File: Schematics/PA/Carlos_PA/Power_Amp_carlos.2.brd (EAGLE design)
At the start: 70.2 x 70.2 mm, 107 parts, among them J1 4_PIN_AMPCONN, U1 LME49830, U2 LME49830, U3 LME49830

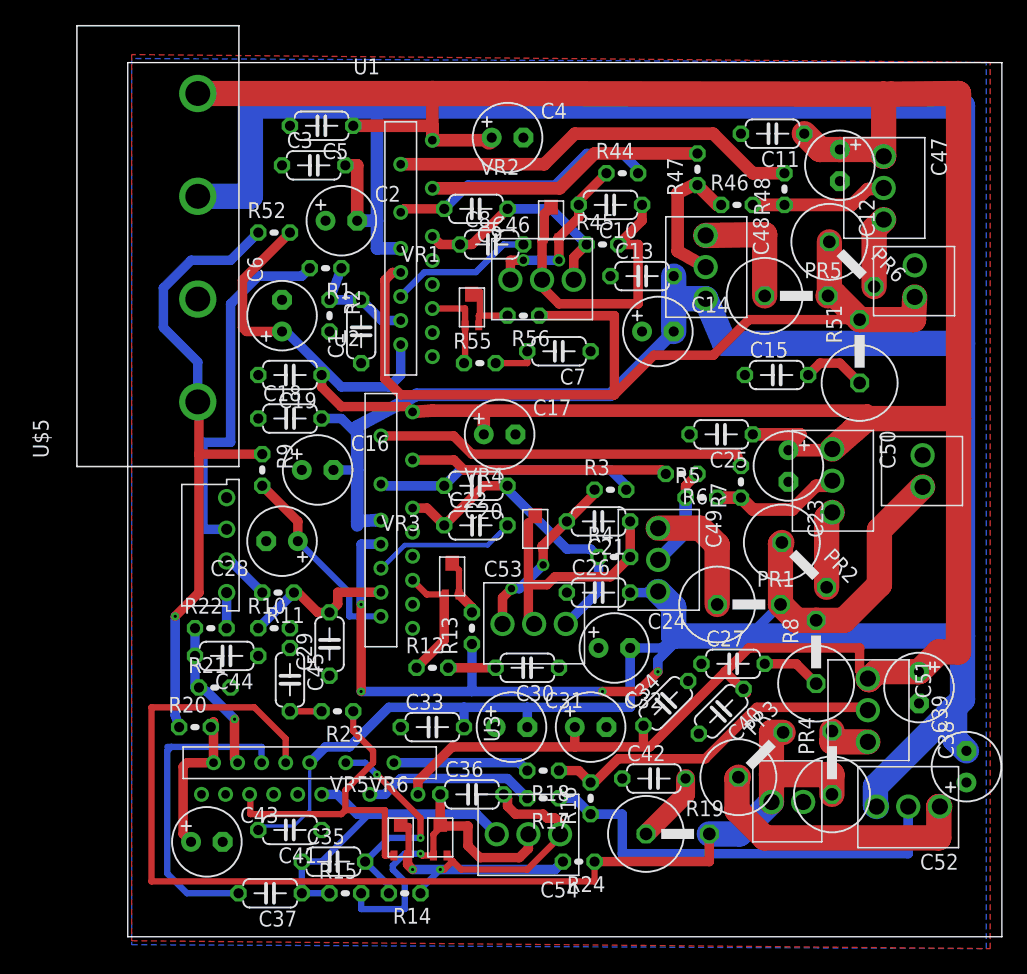
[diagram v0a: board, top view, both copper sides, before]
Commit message: updating to master
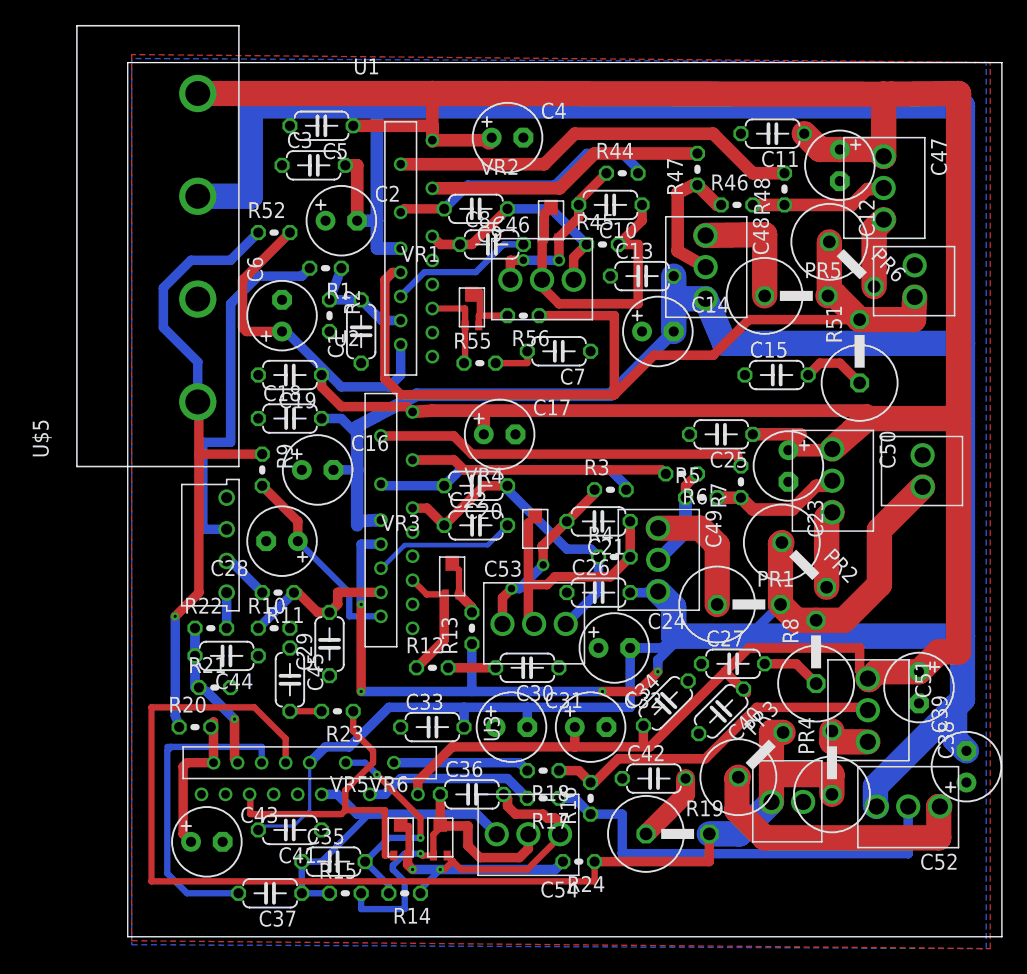
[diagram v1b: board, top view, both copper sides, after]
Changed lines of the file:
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@@
 <setting verticaltext="up"/>
 </settings>
-<grid distance="0.003125" unitdist="mic" unit="inch" style="lines" multiple="1" display="no" altdistance="0.025" altunitdist="inch" altunit="inch"/>
+<grid distance="0.01" unitdist="inch" unit="inch" style="lines" multiple="1" display="yes" altdistance="0.025" altunitdist="inch" altunit="inch"/>
 <layers>
-<layer number="1" name="Top" color="4" fill="1" visible="yes" active="yes"/>
+<layer number="1" name="Top" color="4" fill="1" visible="no" active="yes"/>
 <layer number="16" name="Bottom" color="1" fill="1" visible="yes" active="yes"/>
 <layer number="17" name="Pads" color="2" fill="1" visible="yes" active="yes"/>
@@
 <layer number="19" name="Unrouted" color="6" fill="1" visible="yes" active="yes"/>
 <layer number="20" name="Dimension" color="15" fill="1" visible="yes" active="yes"/>
-<layer number="21" name="tPlace" color="7" fill="1" visible="yes" active="yes"/>
+<layer number="21" name="tPlace" color="7" fill="1" visible="no" active="yes"/>
 <layer number="22" name="bPlace" color="7" fill="1" visible="yes" active="yes"/>
 <layer number="23" name="tOrigins" color="15" fill="1" visible="yes" active="yes"/>
 <layer number="24" name="bOrigins" color="15" fill="1" visible="yes" active="yes"/>
-<layer number="25" name="tNames" color="7" fill="1" visible="yes" active="yes"/>
+<layer number="25" name="tNames" color="7" fill="1" visible="no" active="yes"/>
 <layer number="26" name="bNames" color="7" fill="1" visible="yes" active="yes"/>
 <layer number="27" name="tValues" color="7" fill="1" visible="no" active="yes"/>
@@
 </class>
 </classes>
-<designrules name="default">
-<description language="de">&lt;b&gt;EAGLE Design Rules&lt;/b&gt;
+<designrules name="epl-lpkf">
+<description language="en">&lt;b&gt;EAGLE Design Rules for PSU Electronics Prototyping Lab&lt;/b&gt;
 &lt;p&gt;
-Die Standard-Design-Rules sind so gewählt, dass sie für
-die meisten Anwendungen passen. Sollte ihre Platine
-besondere Anforderungen haben, treffen Sie die erforderlichen
-Einstellungen hier und speichern die Design Rules unter
-einem neuen Namen ab.</description>
-<description language="en">&lt;b&gt;EAGLE Design Rules&lt;/b&gt;
-&lt;p&gt;
-The default Design Rules have been set to cover
-a wide range of applications. Your particular design
-may have different requirements, so please make the
-necessary adjustments and save your customized
-design rules under a new name.</description>
+2013-03-03: Modified from  &lt;b&gt;sunstone_quickturn.dru&lt;/b&gt; to meet minimum drills and spacing for the LPKF S63 Circuit Board Router.
+&lt;/p&gt;</description>
 <param name="layerSetup" value="(1*16)"/>
-<param name="mtCopper" value="0.035mm 0.035mm 0.035mm 0.035mm 0.035mm 0.035mm 0.035mm 0.035mm 0.035mm 0.035mm 0.035mm 0.035mm 0.035mm 0.035mm 0.035mm 0.035mm"/>
-<param name="mtIsolate" value="1.5mm 0.15mm 0.2mm 0.15mm 0.2mm 0.15mm 0.2mm 0.15mm 0.2mm 0.15mm 0.2mm 0.15mm 0.2mm 0.15mm 0.2mm"/>
+<param name="mtCopper" value="0.0178mm 0.0356mm 0.0356mm 0.0356mm 0.0356mm 0.0356mm 0.0356mm 0.0356mm 0.0356mm 0.0356mm 0.0356mm 0.0356mm 0.0356mm 0.0356mm 0.0356mm 0.0178mm"/>
+<param name="mtIsolate" value="59mil 0.1499mm 0.2007mm 0.1499mm 0.2007mm 0.1499mm 0.2007mm 0.1499mm 0.2007mm 0.1499mm 0.2007mm 0.1499mm 0.2007mm 0.1499mm 0.2007mm"/>
 <param name="mdWireWire" value="8mil"/>
 <param name="mdWirePad" value="8mil"/>
@@
 <param name="mdViaViaSameLayer" value="8mil"/>
 <param name="mnLayersViaInSmd" value="2"/>
-<param name="mdCopperDimension" value="40mil"/>
-<param name="mdDrill" value="8mil"/>
+<param name="mdCopperDimension" value="15mil"/>
+<param name="mdDrill" value="15mil"/>
 <param name="mdSmdStop" value="0mil"/>
-<param name="msWidth" value="10mil"/>
-<param name="msDrill" value="24mil"/>
-<param name="msMicroVia" value="9.99mm"/>
+<param name="msWidth" value="8mil"/>
+<param name="msDrill" value="0.35mm"/>
+<param name="msMicroVia" value="9.9898mm"/>
 <param name="msBlindViaRatio" value="0.5"/>
 <param name="rvPadTop" value="0.25"/>
@@
 <param name="rvMicroViaOuter" value="0.25"/>
 <param name="rvMicroViaInner" value="0.25"/>
-<param name="rlMinPadTop" value="10mil"/>
-<param name="rlMaxPadTop" value="20mil"/>
-<param name="rlMinPadInner" value="10mil"/>
-<param name="rlMaxPadInner" value="20mil"/>
-<param name="rlMinPadBottom" value="10mil"/>
-<param name="rlMaxPadBottom" value="20mil"/>
+<param name="rlMinPadTop" value="8mil"/>
+<param name="rlMaxPadTop" value="999mil"/>
+<param name="rlMinPadInner" value="0mil"/>
+<param name="rlMaxPadInner" value="0mil"/>
+<param name="rlMinPadBottom" value="8mil"/>
+<param name="rlMaxPadBottom" value="999mil"/>
 <param name="rlMinViaOuter" value="8mil"/>
-<param name="rlMaxViaOuter" value="20mil"/>
-<param name="rlMinViaInner" value="8mil"/>
-<param name="rlMaxViaInner" value="20mil"/>
-<param name="rlMinMicroViaOuter" value="4mil"/>
-<param name="rlMaxMicroViaOuter" value="20mil"/>
-<param name="rlMinMicroViaInner" value="4mil"/>
-<param name="rlMaxMicroViaInner" value="20mil"/>
+<param name="rlMaxViaOuter" value="999mil"/>
+<param name="rlMinViaInner" value="0mil"/>
+<param name="rlMaxViaInner" value="0mil"/>
+<param name="rlMinMicroViaOuter" value="8mil"/>
+<param name="rlMaxMicroViaOuter" value="999mil"/>
+<param name="rlMinMicroViaInner" value="0mil"/>
+<param name="rlMaxMicroViaInner" value="0mil"/>
 <param name="psTop" value="-1"/>
 <param name="psBottom" value="-1"/>
@@
 <param name="mvStopFrame" value="1"/>
 <param name="mvCreamFrame" value="0"/>
-<param name="mlMinStopFrame" value="4mil"/>
-<param name="mlMaxStopFrame" value="4mil"/>
+<param name="mlMinStopFrame" value="3mil"/>
+<param name="mlMaxStopFrame" value="3mil"/>
 <param name="mlMinCreamFrame" value="0mil"/>
 <param name="mlMaxCreamFrame" value="0mil"/>
@@
 <param name="checkRestrict" value="1"/>
 <param name="useDiameter" value="13"/>
-<param name="maxErrors" value="50"/>
+<param name="maxErrors" value="500"/>
 </designrules>
 <autorouter>
@@
 <contactref element="U$7" pad="P$2"/>
 <contactref element="U$8" pad="P$2"/>
-<wire x1="21.185" y1="12.3825" x2="21.59" y2="20.955" width="0" layer="19" extent="1-1"/>
 </signal>
 <signal name="V-">
